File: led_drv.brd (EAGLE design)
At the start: 30 x 20 mm, 20 parts, among them Q1 FDD5612, U1 NCS20071, U2 TPS70950

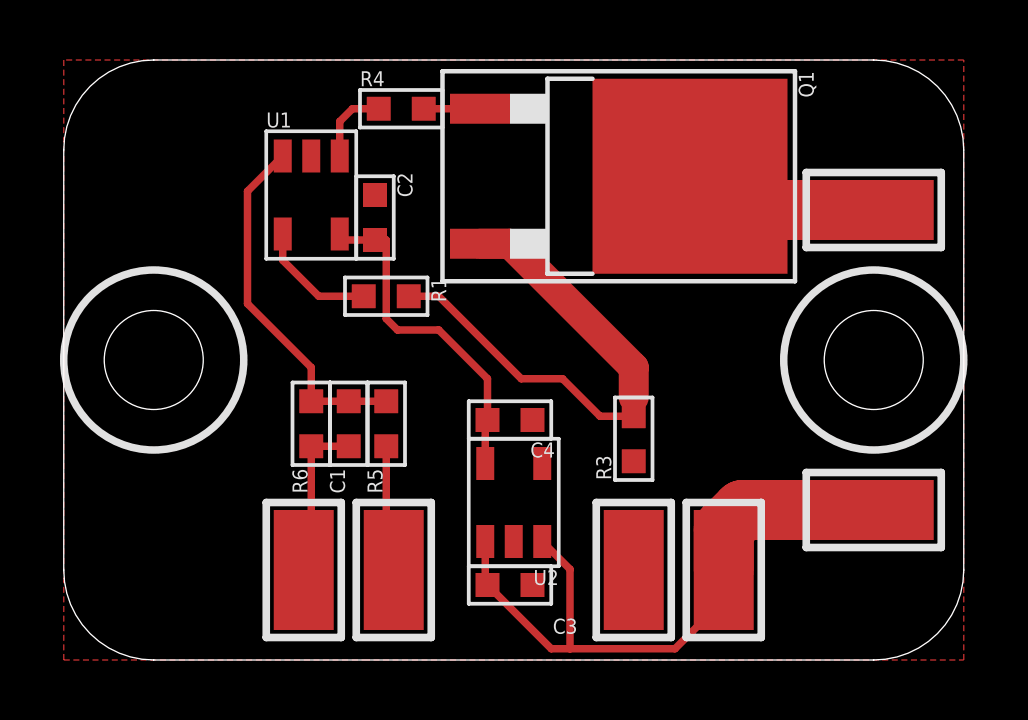
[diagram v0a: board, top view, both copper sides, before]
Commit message: ESP32 added with architecture implemented. First attempt.
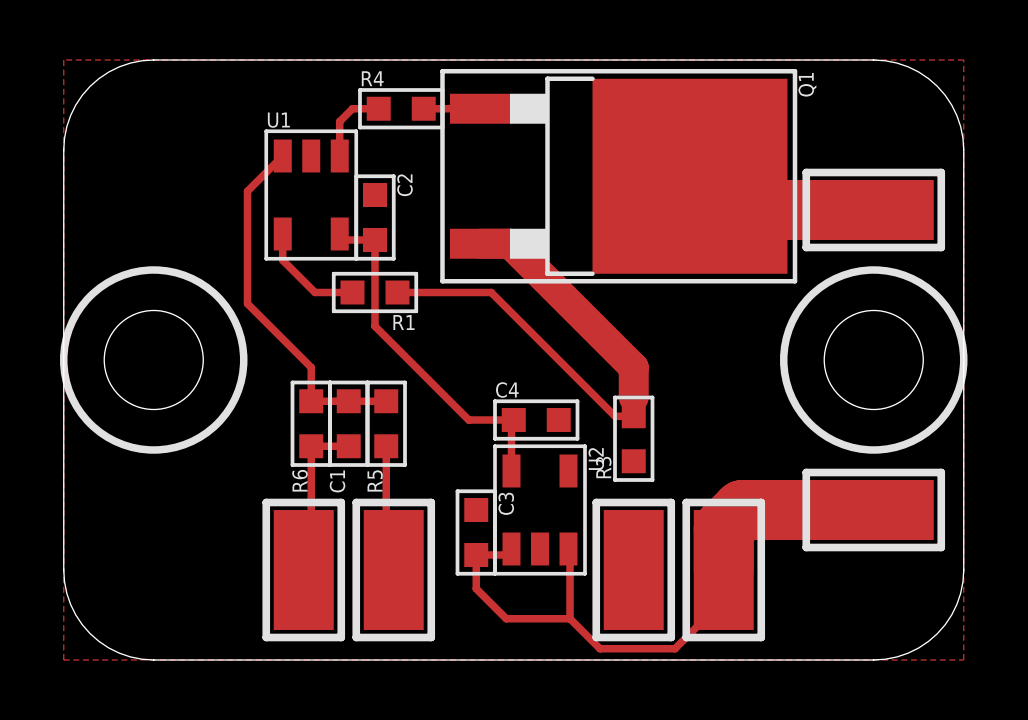
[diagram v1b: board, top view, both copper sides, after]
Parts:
- moved C3 2.08 mm to (-1.25, -5.75), turned to 270 degrees
- moved U2 0.91 mm to (0.88, -5.00)
- moved C4 0.88 mm to (0.75, -2.00)
- moved R1 0.40 mm to (-4.62, 2.25)
